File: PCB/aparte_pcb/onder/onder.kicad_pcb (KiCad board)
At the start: 2 copper layers, 170 x 170 mm, 77 parts, among them J1 Conn_01x04_Socket, J2 Conn_01x10_Socket, J3 Screw_Terminal_01x01, J4 Screw_Terminal_01x01, J5 Screw_Terminal_01x01, Q1 NPN, Q2 NPN, Q3 NPN

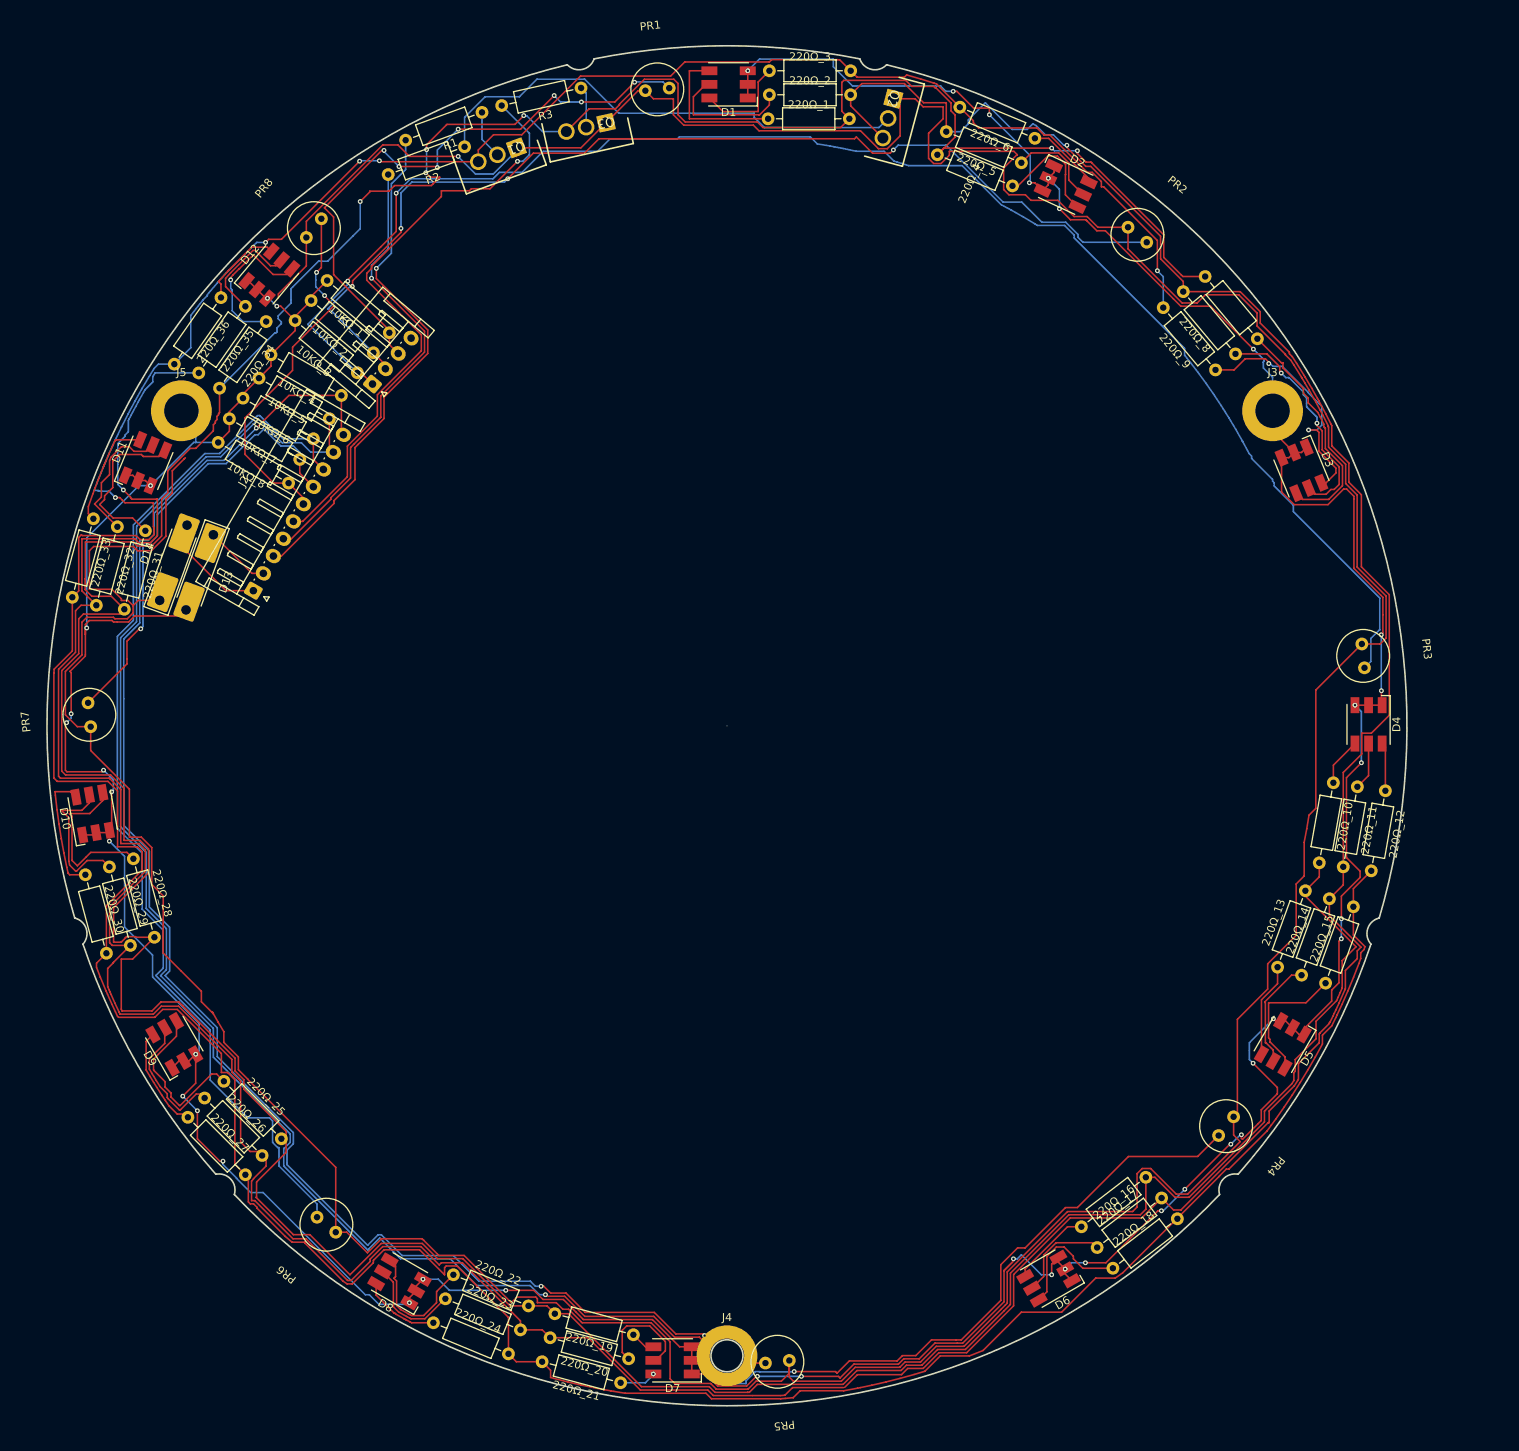
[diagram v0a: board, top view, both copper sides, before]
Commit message: pcb pre autoroute upload
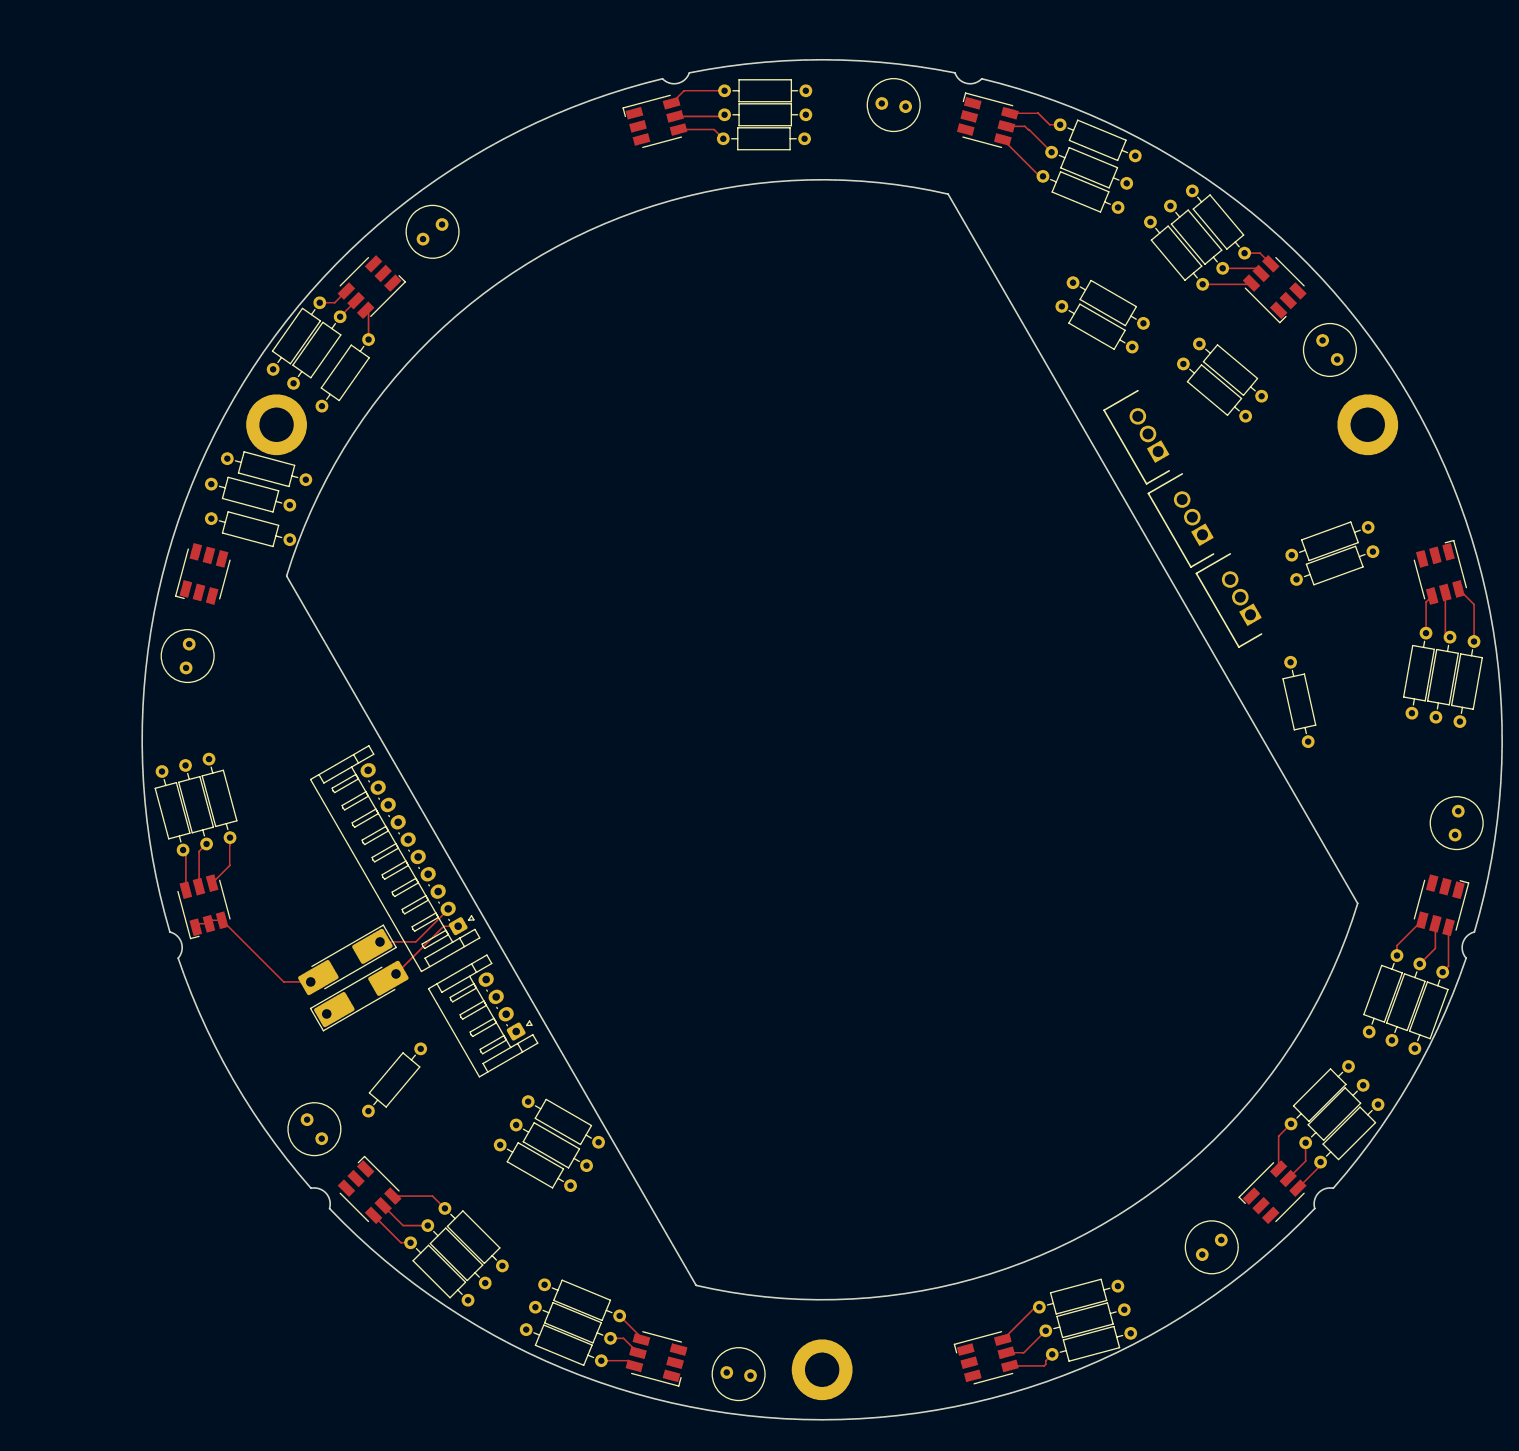
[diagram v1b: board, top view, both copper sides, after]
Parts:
- moved R2 124.3 mm to (184.9, 80.6)
- moved R1 122.3 mm to (184.3, 77.6)
- moved R3 122.2 mm to (176.8, 104.4), turned to 102.5 degrees
- moved 10KΩ_2 111.2 mm to (171.0, 61.2)
- moved 10KΩ_3 111.2 mm to (169.0, 63.7)
- moved 10KΩ_8 106.8 mm to (154.9, 55.0)
- moved 10KΩ_7 106.8 mm to (156.3, 52.1)
- moved Q3 101.4 mm to (169.6, 88.5), turned to 120 degrees
- moved 10KΩ_5 98.7 mm to (86.6, 157.4)
- moved 10KΩ_6 98.7 mm to (84.6, 159.9)
- moved 10KΩ_4 98.7 mm to (88.1, 154.4)
- moved Q1 98.5 mm to (163.6, 78.5), turned to 120 degrees
- moved 10KΩ_1 89.6 mm to (65.9, 142.8), turned to -130 degrees
- moved J1 82.9 mm to (77.8, 140.6), turned to 120 degrees
- moved D14 58.8 mm to (58.5, 135.9), turned to 30 degrees
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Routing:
- net Net-(D14-K): track 585.4 -> 0.00 mm, vias 1 -> 0
- net Net-(D1-BK): track 575.0 -> 17.9 mm, vias 41 -> 0
- net Net-(Q3-E): track 540.8 -> 0.00 mm, vias 6 -> 0
- net Net-(Q2-E): track 513.9 -> 0.00 mm, vias 2 -> 0
- net Net-(Q1-E): track 508.5 -> 0.00 mm, vias 5 -> 0
- net pr4: track 274.9 -> 0.00 mm, vias 4 -> 0
- net pr5: track 201.9 -> 0.00 mm, vias 1 -> 0
- net pr3: track 193.9 -> 0.00 mm, vias 2 -> 0
- net pr6: track 133.8 -> 0.00 mm
- net pr2: track 131.7 -> 0.00 mm, vias 4 -> 0
- net pr1: track 76.0 -> 0.00 mm, vias 7 -> 0
- net ROOD: track 75.8 -> 0.00 mm, vias 1 -> 0
- net BLAUW: track 64.8 -> 0.00 mm, vias 1 -> 0
- net Net-(Q2-B): track 61.9 -> 0.00 mm
- net GROEN: track 57.0 -> 0.00 mm, vias 1 -> 0
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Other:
- outline, holes or cut-outs redrawn
